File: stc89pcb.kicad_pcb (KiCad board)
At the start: 2 copper layers, 57.2 x 26.2 mm, 20 parts, among them J1 USB_C_Receptacle_USB2.0_16P, J2 Conn_01x22_Pin, J3 Conn_01x22_Pin, SW1 TS-1088-AR02016, SW2 TA-3531S-A2, U1 STC89C52RC-40I_C8707, U2 CH340C, X1 X322512MSB4SI

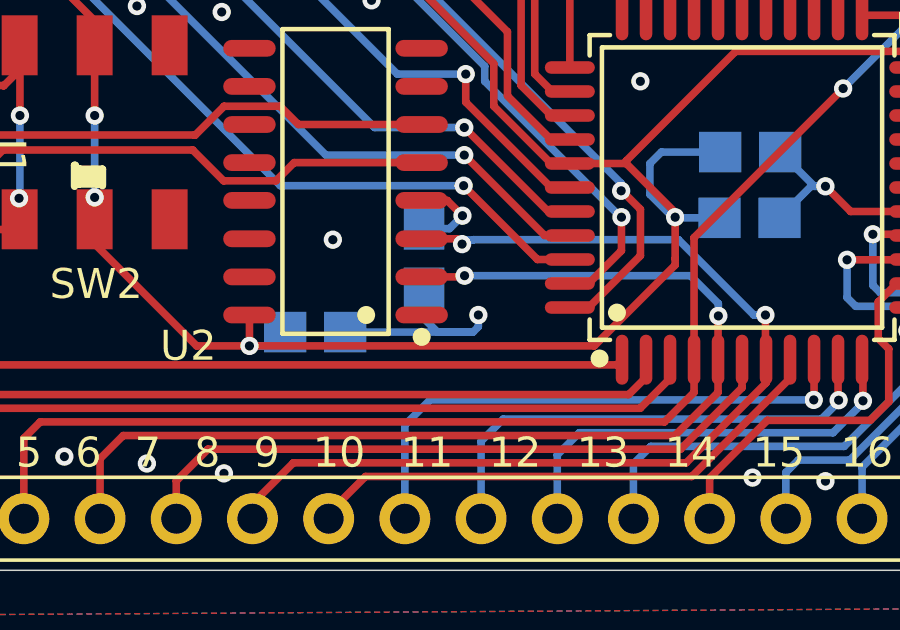
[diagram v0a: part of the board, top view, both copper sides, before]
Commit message: 2
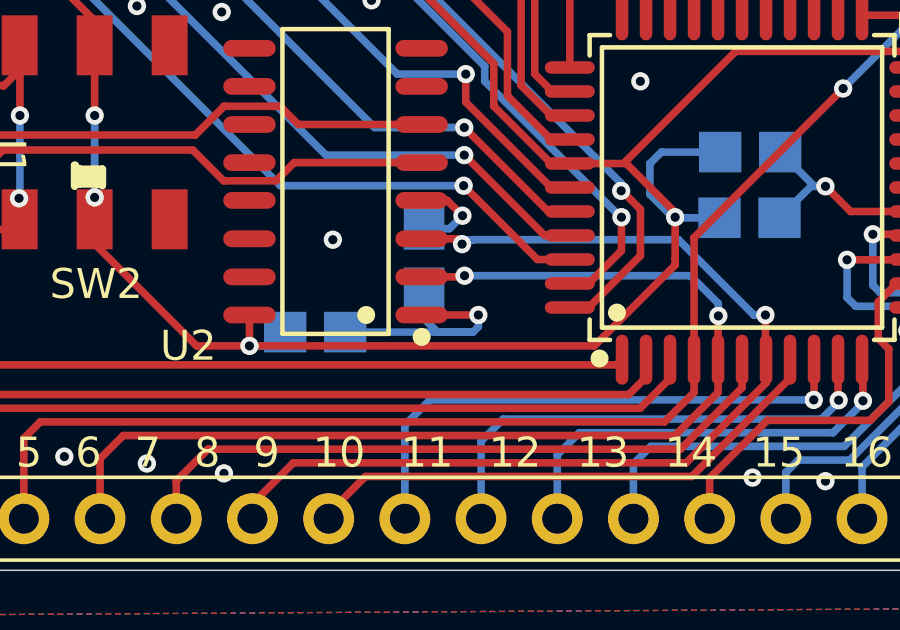
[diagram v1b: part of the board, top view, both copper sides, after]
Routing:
- net GND: track 70.1 -> 72.0 mm
